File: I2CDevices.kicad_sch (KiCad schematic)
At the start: 37 parts, among them Q20 IRLML2803, Q21 SiRA99DP, U1 OPT4003DNPRQ1, U2 PCA9633DP2, U4 DRV8235RTER

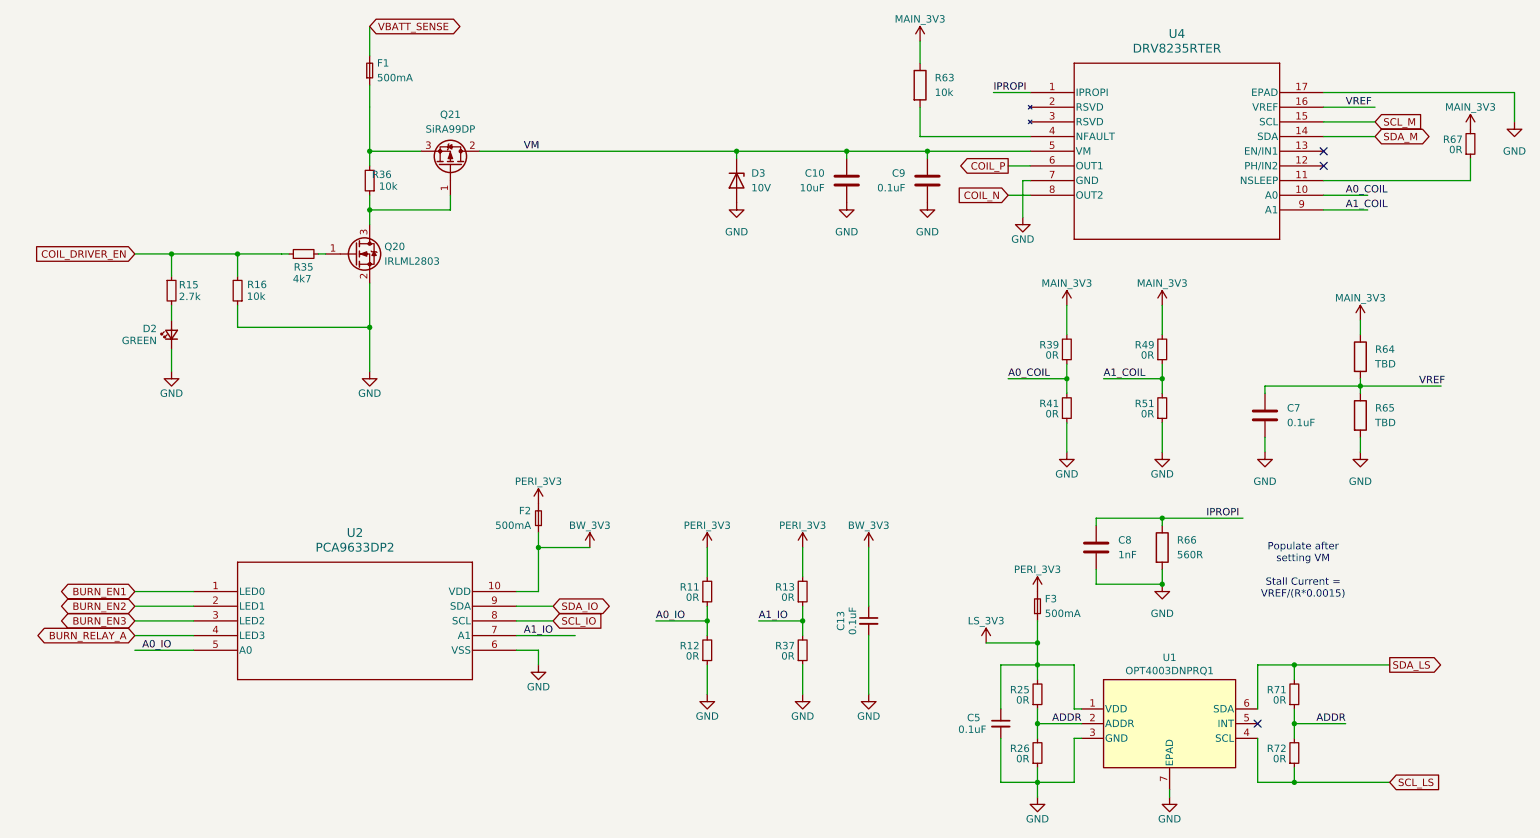
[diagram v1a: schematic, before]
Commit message: Stash
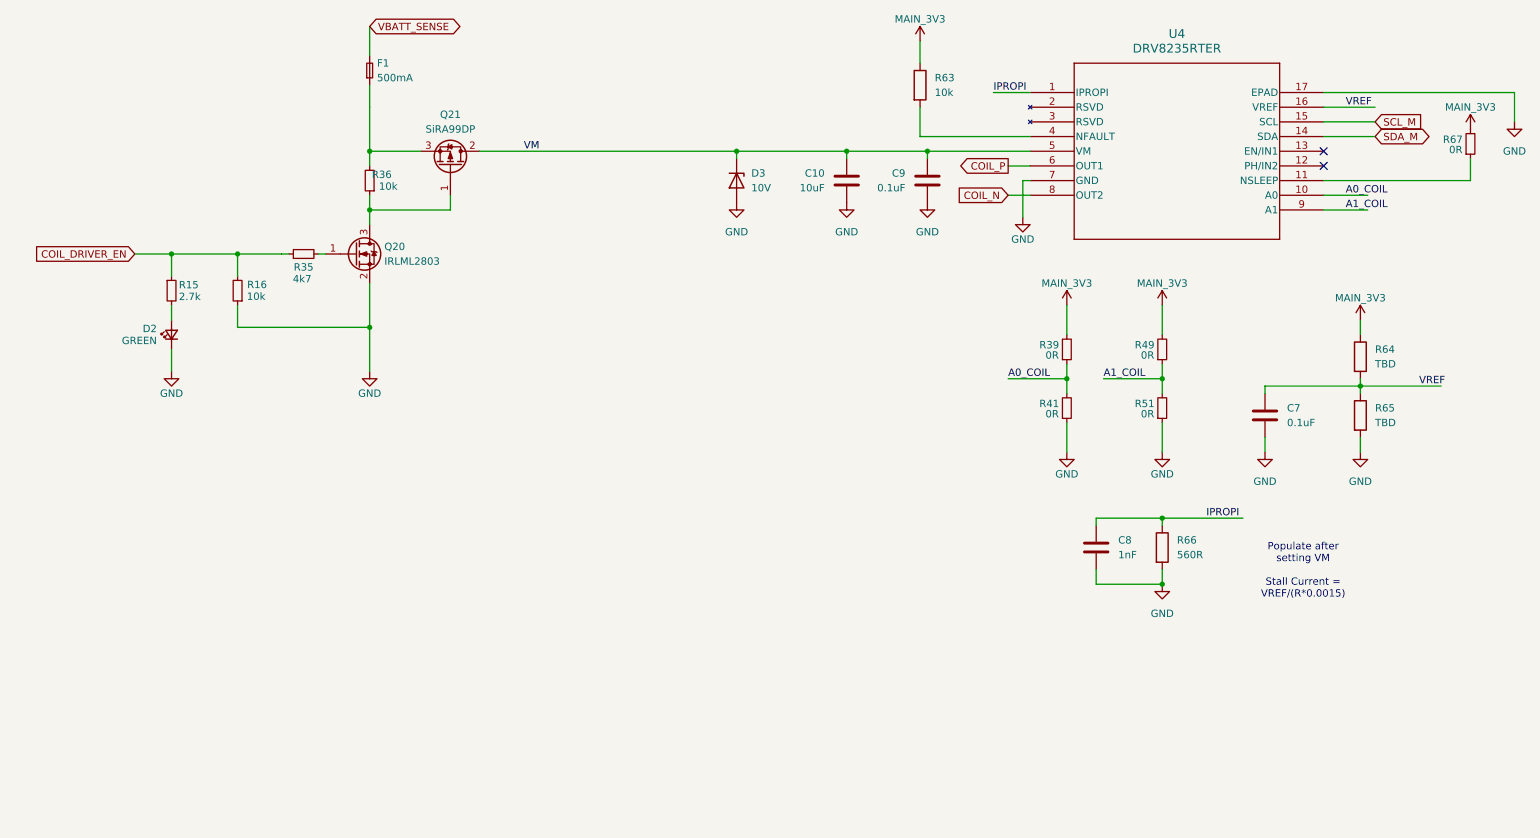
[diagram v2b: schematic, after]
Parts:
- removed C13, C5: 0.1uF, Capacitor_SMD:C_0603_1608Metric, symbol Device:C_Small
- removed F2, F3: 500mA, Fuse:Fuse_0603_1608Metric, symbol Device:Fuse_Small
- removed R11, R12, R13, R25, R26, R37, R71, R72: 0R, Resistor_SMD:R_0603_1608Metric, symbol Device:R_Small
- removed U1: OPT4003DNPRQ1, Argus-IC:OPT4003, symbol Argus-IC:OPT4003DNPRQ1
- removed U2: PCA9633DP2, Argus-IC:SOT552-1_NXP, symbol Argus-IC:PCA9633DP2
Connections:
- no-connect marks 3 -> 2
